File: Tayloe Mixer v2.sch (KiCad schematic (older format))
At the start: 38 parts, among them J1 BNC, J2 Pad, J3 Audio_Jack, J4 Conn_01x04_Female, J5 Pad, T1 6:31, T2 31:6, T3 T50_SPLITTER, U1 LM7805_TO220, U2 FST3253, U3 LM358, U4 si5351, U5 LD33V

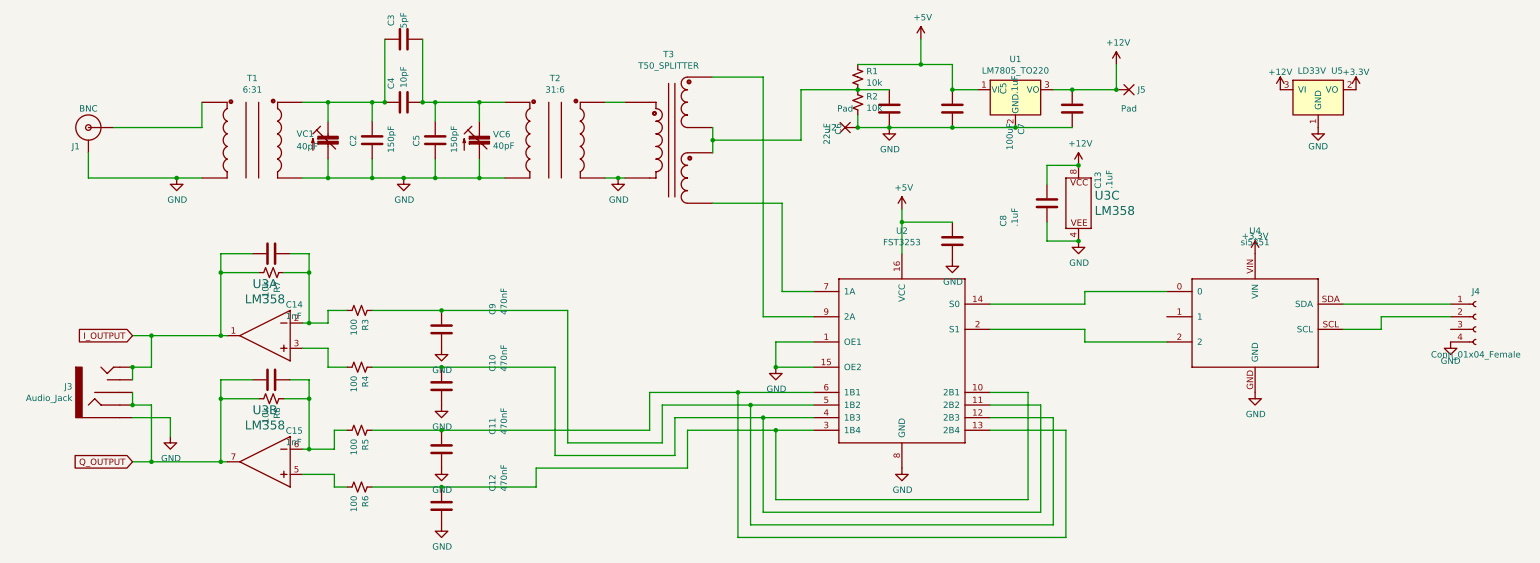
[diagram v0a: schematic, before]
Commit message: gg
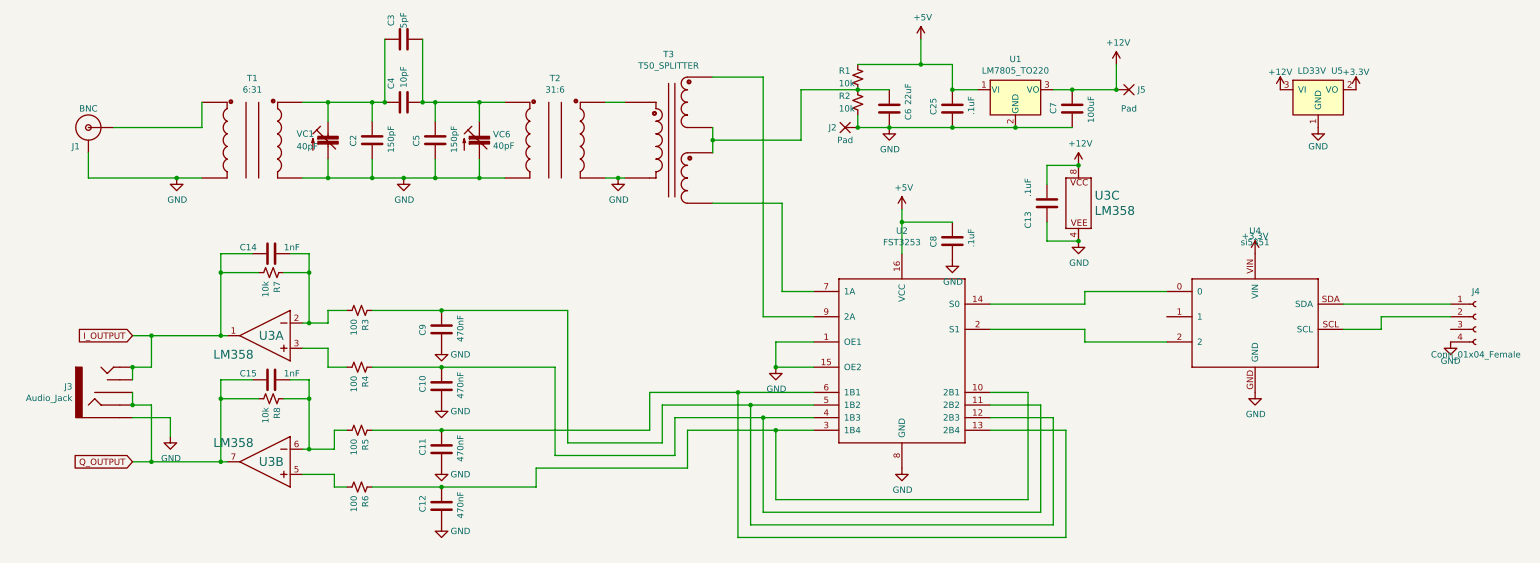
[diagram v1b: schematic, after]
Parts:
- renumbered C5 to C25
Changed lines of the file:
@@
 U 1 1 5E9FAC03
 P 8200 1750
-F 0 "R1" H 8268 1796 50  0000 L CNN
-F 1 "10k" H 8268 1705 50  0000 L CNN
+F 0 "R1" H 8050 1800 50  0000 L CNN
+F 1 "10k" H 8050 1700 50  0000 L CNN
 F 2 "Xenir:Capacitor 0805" H 8200 1750 50  0001 C CNN
 F 3 "~" H 8200 1750 50  0001 C CNN
@@
 U 1 1 5E9FB5EE
 P 8200 1950
-F 0 "R2" H 8268 1996 50  0000 L CNN
-F 1 "10k" H 8268 1905 50  0000 L CNN
+F 0 "R2" H 8050 2000 50  0000 L CNN
+F 1 "10k" H 8050 1900 50  0000 L CNN
 F 2 "Xenir:Capacitor 0805" H 8200 1950 50  0001 C CNN
 F 3 "~" H 8200 1950 50  0001 C CNN
@@
 $EndComp
 $Comp
-L Xenir:Capacitor C5
+L Xenir:Capacitor C25
 U 1 1 5E9FBB07
 P 8950 2000
-F 0 "C5" H 9065 1596 50  0000 L CNN
-F 1 ".1uF" H 9065 1505 50  0000 L CNN
+F 0 "C25" H 8900 2150 50  0000 L CNN
+F 1 ".1uF" H 8900 1850 50  0000 L CNN
 F 2 "Xenir:Capacitor 1206" H 8950 2000 50  0001 C CNN
 F 3 "" H 8950 2000 50  0001 C CNN
@@
 U 1 1 5EA05D6A
 P 9900 2000
-F 0 "C7" H 10015 1596 50  0000 L CNN
-F 1 "100uF" H 10015 1505 50  0000 L CNN
+F 0 "C7" H 9850 1850 50  0000 L CNN
+F 1 "100uF" H 9800 2150 50  0000 L CNN
 F 2 "Capacitor_SMD:CP_Elec_6.3x5.4" H 9900 2000 50  0001 C CNN
 F 3 "" H 9900 2000 50  0001 C CNN
@@
 U 1 1 5EA063C0
 P 8450 2000
-F 0 "C6" H 8565 1596 50  0000 L CNN
-F 1 "22uF" H 8565 1505 50  0000 L CNN
+F 0 "C6" H 8450 2150 50  0000 L CNN
+F 1 "22uF" H 8250 2150 50  0000 L CNN
 F 2 "Capacitor_SMD:CP_Elec_4x5.4" H 8450 2000 50  0001 C CNN
 F 3 "" H 8450 2000 50  0001 C CNN
@@
 U 1 1 5EA383DE
 P 8950 3050
-F 0 "C8" H 9065 2646 50  0000 L CNN
-F 1 ".1uF" H 9065 2555 50  0000 L CNN
+F 0 "C8" H 8900 3200 50  0000 L CNN
+F 1 ".1uF" H 8900 2900 50  0000 L CNN
 F 2 "Xenir:Capacitor 1206" H 8950 3050 50  0001 C CNN
 F 3 "" H 8950 3050 50  0001 C CNN
@@
 U 1 1 5EA6792B
 P 4900 3750
-F 0 "C9" H 5015 3346 50  0000 L CNN
-F 1 "470nF" H 5015 3255 50  0000 L CNN
+F 0 "C9" H 4850 3900 50  0000 L CNN
+F 1 "470nF" H 4800 3600 50  0000 L CNN
 F 2 "Xenir:Capacitor 0805" H 4900 3750 50  0001 C CNN
 F 3 "" H 4900 3750 50  0001 C CNN
@@
 U 1 1 5EA68A05
 P 4900 4200
-F 0 "C10" H 5015 3796 50  0000 L CNN
-F 1 "470nF" H 5015 3705 50  0000 L CNN
+F 0 "C10" H 4850 4350 50  0000 L CNN
+F 1 "470nF" H 4800 4050 50  0000 L CNN
 F 2 "Xenir:Capacitor 0805" H 4900 4200 50  0001 C CNN
 F 3 "" H 4900 4200 50  0001 C CNN
@@
 U 1 1 5EA6950B
 P 4900 4700
-F 0 "C11" H 5015 4296 50  0000 L CNN
-F 1 "470nF" H 5015 4205 50  0000 L CNN
+F 0 "C11" H 4850 4850 50  0000 L CNN
+F 1 "470nF" H 4800 4550 50  0000 L CNN
 F 2 "Xenir:Capacitor 0805" H 4900 4700 50  0001 C CNN
 F 3 "" H 4900 4700 50  0001 C CNN
@@
 U 1 1 5EA69901
 P 4900 5150
-F 0 "C12" H 5015 4746 50  0000 L CNN
-F 1 "470nF" H 5015 4655 50  0000 L CNN
+F 0 "C12" H 4850 5300 50  0000 L CNN
+F 1 "470nF" H 4800 5000 50  0000 L CNN
 F 2 "Xenir:Capacitor 0805" H 4900 5150 50  0001 C CNN
 F 3 "" H 4900 5150 50  0001 C CNN
@@
 P 4900 3900
 F 0 "#PWR05" H 4900 3650 50  0001 C CNN
-F 1 "GND" H 4905 3727 50  0000 C CNN
+F 1 "GND" H 5050 3850 50  0000 C CNN
 F 2 "" H 4900 3900 50  0001 C CNN
 F 3 "" H 4900 3900 50  0001 C CNN
@@
 P 4900 4350
 F 0 "#PWR06" H 4900 4100 50  0001 C CNN
-F 1 "GND" H 4905 4177 50  0000 C CNN
+F 1 "GND" H 5050 4300 50  0000 C CNN
 F 2 "" H 4900 4350 50  0001 C CNN
 F 3 "" H 4900 4350 50  0001 C CNN
@@
 P 4900 4850
 F 0 "#PWR07" H 4900 4600 50  0001 C CNN
-F 1 "GND" H 4905 4677 50  0000 C CNN
+F 1 "GND" H 5050 4800 50  0000 C CNN
 F 2 "" H 4900 4850 50  0001 C CNN
 F 3 "" H 4900 4850 50  0001 C CNN
@@
 P 4900 5300
 F 0 "#PWR08" H 4900 5050 50  0001 C CNN
-F 1 "GND" H 4905 5127 50  0000 C CNN
+F 1 "GND" H 5050 5250 50  0000 C CNN
 F 2 "" H 4900 5300 50  0001 C CNN
 F 3 "" H 4900 5300 50  0001 C CNN
@@
 U 1 1 5EA9F5A6
 P 3500 3800
-F 0 "U3" H 3500 4210 70  0000 C CNN
-F 1 "LM358" H 3500 4089 70  0000 C CNN
+F 0 "U3" H 3450 3800 70  0000 C CNN
+F 1 "LM358" H 3750 3650 70  0000 C CNN
 F 2 "Xenir:SOIC8" H 3450 3750 50  0001 C CNN
 F 3 "" H 3450 3750 50  0001 C CNN
@@
 U 2 1 5EAA17EF
 P 3500 4800
-F 0 "U3" H 3500 5210 70  0000 C CNN
-F 1 "LM358" H 3500 5089 70  0000 C CNN
+F 0 "U3" H 3450 4800 70  0000 C CNN
+F 1 "LM358" H 3750 4950 70  0000 C CNN
 F 2 "Xenir:SOIC8" H 3450 4750 50  0001 C CNN
 F 3 "" H 3450 4750 50  0001 C CNN
@@
 U 1 1 5EAC8FB2
 P 9700 2750
-F 0 "C13" H 9815 2346 50  0000 L CNN
-F 1 ".1uF" H 9815 2255 50  0000 L CNN
+F 0 "C13" H 9500 2900 50  0000 L CNN
+F 1 ".1uF" H 9750 2900 50  0000 L CNN
 F 2 "Xenir:Capacitor 1206" H 9700 2750 50  0001 C CNN
 F 3 "" H 9700 2750 50  0001 C CNN
@@
 U 1 1 5EADF0CD
 P 3550 4150
-F 0 "C15" H 3665 3746 50  0000 L CNN
-F 1 "1nF" H 3665 3655 50  0000 L CNN
+F 0 "C15" H 3300 4200 50  0000 L CNN
+F 1 "1nF" H 3650 4200 50  0000 L CNN
 F 2 "Xenir:Capacitor 0805" H 3550 4150 50  0001 C CNN
 F 3 "" H 3550 4150 50  0001 C CNN
@@
 U 1 1 5EADE1CD
 P 3550 3150
-F 0 "C14" H 3665 2746 50  0000 L CNN
-F 1 "1nF" H 3665 2655 50  0000 L CNN
+F 0 "C14" H 3300 3200 50  0000 L CNN
+F 1 "1nF" H 3650 3200 50  0000 L CNN
 F 2 "Xenir:Capacitor 0805" H 3550 3150 50  0001 C CNN
 F 3 "" H 3550 3150 50  0001 C CNN
@@
 P 8100 2000
 F 0 "J2" H 8000 1850 50  0000 C CNN
-F 1 "Pad" H 8100 2000 50  0000 C CNN
+F 1 "Pad" H 8100 1750 50  0000 C CNN
 F 2 "Xenir:Pad" H 8100 2000 50  0001 C CNN
 F 3 "" H 8100 2000 50  0001 C CNN

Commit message: gg
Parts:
- R1, R2, R3, R4, R5, R6, R7, R8: footprint Xenir:Capacitor 0805 -> Xenir:Resistor 0805
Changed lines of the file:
@@
 F 0 "R1" H 8050 1800 50  0000 L CNN
 F 1 "10k" H 8050 1700 50  0000 L CNN
-F 2 "Xenir:Capacitor 0805" H 8200 1750 50  0001 C CNN
+F 2 "Xenir:Resistor 0805" H 8200 1750 50  0001 C CNN
 F 3 "~" H 8200 1750 50  0001 C CNN
 	1    8200 1750
@@
 F 0 "R2" H 8050 2000 50  0000 L CNN
 F 1 "10k" H 8050 1900 50  0000 L CNN
-F 2 "Xenir:Capacitor 0805" H 8200 1950 50  0001 C CNN
+F 2 "Xenir:Resistor 0805" H 8200 1950 50  0001 C CNN
 F 3 "~" H 8200 1950 50  0001 C CNN
 	1    8200 1950
@@
 F 0 "R3" H 4318 3646 50  0000 L CNN
 F 1 "100" H 4318 3555 50  0000 L CNN
-F 2 "Xenir:Capacitor 0805" H 4250 3600 50  0001 C CNN
+F 2 "Xenir:Resistor 0805" H 4250 3600 50  0001 C CNN
 F 3 "~" H 4250 3600 50  0001 C CNN
 	1    4250 3600
@@
 F 0 "R4" H 4318 4096 50  0000 L CNN
 F 1 "100" H 4318 4005 50  0000 L CNN
-F 2 "Xenir:Capacitor 0805" H 4250 4050 50  0001 C CNN
+F 2 "Xenir:Resistor 0805" H 4250 4050 50  0001 C CNN
 F 3 "~" H 4250 4050 50  0001 C CNN
 	1    4250 4050
@@
 F 0 "R5" H 4318 4596 50  0000 L CNN
 F 1 "100" H 4318 4505 50  0000 L CNN
-F 2 "Xenir:Capacitor 0805" H 4250 4550 50  0001 C CNN
+F 2 "Xenir:Resistor 0805" H 4250 4550 50  0001 C CNN
 F 3 "~" H 4250 4550 50  0001 C CNN
 	1    4250 4550
@@
 F 0 "R6" H 4318 5046 50  0000 L CNN
 F 1 "100" H 4318 4955 50  0000 L CNN
-F 2 "Xenir:Capacitor 0805" H 4250 5000 50  0001 C CNN
+F 2 "Xenir:Resistor 0805" H 4250 5000 50  0001 C CNN
 F 3 "~" H 4250 5000 50  0001 C CNN
 	1    4250 5000
@@
 F 0 "R7" H 3618 3346 50  0000 L CNN
 F 1 "10k" H 3618 3255 50  0000 L CNN
-F 2 "Xenir:Capacitor 0805" H 3550 3300 50  0001 C CNN
+F 2 "Xenir:Resistor 0805" H 3550 3300 50  0001 C CNN
 F 3 "~" H 3550 3300 50  0001 C CNN
 	1    3550 3300
@@
 F 0 "R8" H 3618 4346 50  0000 L CNN
 F 1 "10k" H 3618 4255 50  0000 L CNN
-F 2 "Xenir:Capacitor 0805" H 3550 4300 50  0001 C CNN
+F 2 "Xenir:Resistor 0805" H 3550 4300 50  0001 C CNN
 F 3 "~" H 3550 4300 50  0001 C CNN
 	1    3550 4300

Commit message: rescue
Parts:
- C10, C11, C12, C13, C14, C15, C2, C25, C3, C4, C5, C6, C7, C8, C9: symbol Xenir:Capacitor -> Tayloe-Mixer-v2-rescue:Capacitor-Xenir
- J1: symbol Xenir:BNC -> Tayloe-Mixer-v2-rescue:BNC-Xenir
- J2, J5: symbol Xenir:Pad -> Tayloe-Mixer-v2-rescue:Pad-Xenir
- J3: symbol Xenir:Audio_Jack -> Tayloe-Mixer-v2-rescue:Audio_Jack-Xenir
- T1, T2: symbol Xenir:T37_XFRM -> Tayloe-Mixer-v2-rescue:T37_XFRM-Xenir
- T3: symbol Xenir:T50_SPLITTER -> Tayloe-Mixer-v2-rescue:T50_SPLITTER-Xenir
- U2: symbol Xenir:FST3253 -> Tayloe-Mixer-v2-rescue:FST3253-Xenir
- U3: symbol Xenir:LM358 -> Tayloe-Mixer-v2-rescue:LM358-Xenir
- U4: symbol Xenir:si5351 -> Tayloe-Mixer-v2-rescue:si5351-Xenir
- U5: symbol Xenir:LD33V -> Tayloe-Mixer-v2-rescue:LD33V-Xenir
- VC1, VC6: symbol Xenir:Trimcap -> Tayloe-Mixer-v2-rescue:Trimcap-Xenir
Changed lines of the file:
@@
 $EndComp
 $Comp
-L Xenir:Capacitor C25
+L Tayloe-Mixer-v2-rescue:Capacitor-Xenir C25
 U 1 1 5E9FBB07
 P 8950 2000
@@
 	7750 1850 8200 1850
 $Comp
-L Xenir:Capacitor C7
+L Tayloe-Mixer-v2-rescue:Capacitor-Xenir C7
 U 1 1 5EA05D6A
 P 9900 2000
@@
 $EndComp
 $Comp
-L Xenir:Capacitor C6
+L Tayloe-Mixer-v2-rescue:Capacitor-Xenir C6
 U 1 1 5EA063C0
 P 8450 2000
@@
 	8700 1650 8950 1650
 $Comp
-L Xenir:FST3253 U2
+L Tayloe-Mixer-v2-rescue:FST3253-Xenir U2
 U 1 1 5EA318D2
 P 9000 2700
@@
 	8550 2800 8550 2900
 $Comp
-L Xenir:Capacitor C8
+L Tayloe-Mixer-v2-rescue:Capacitor-Xenir C8
 U 1 1 5EA383DE
 P 8950 3050
@@
 	9550 4250 9250 4250
 $Comp
-L Xenir:Capacitor C9
+L Tayloe-Mixer-v2-rescue:Capacitor-Xenir C9
 U 1 1 5EA6792B
 P 4900 3750
@@
 $EndComp
 $Comp
-L Xenir:Capacitor C10
+L Tayloe-Mixer-v2-rescue:Capacitor-Xenir C10
 U 1 1 5EA68A05
 P 4900 4200
@@
 $EndComp
 $Comp
-L Xenir:Capacitor C11
+L Tayloe-Mixer-v2-rescue:Capacitor-Xenir C11
 U 1 1 5EA6950B
 P 4900 4700
@@
 $EndComp
 $Comp
-L Xenir:Capacitor C12
+L Tayloe-Mixer-v2-rescue:Capacitor-Xenir C12
 U 1 1 5EA69901
 P 4900 5150
@@
 $EndComp
 $Comp
-L Xenir:LM358 U3
+L Tayloe-Mixer-v2-rescue:LM358-Xenir U3
 U 1 1 5EA9F5A6
 P 3500 3800
@@
 $EndComp
 $Comp
-L Xenir:LM358 U3
+L Tayloe-Mixer-v2-rescue:LM358-Xenir U3
 U 2 1 5EAA17EF
 P 3500 4800
@@
 $EndComp
 $Comp
-L Xenir:LM358 U3
+L Tayloe-Mixer-v2-rescue:LM358-Xenir U3
 U 3 1 5EAA2951
 P 10050 2750
@@
 $EndComp
 $Comp
-L Xenir:Capacitor C13
+L Tayloe-Mixer-v2-rescue:Capacitor-Xenir C13
 U 1 1 5EAC8FB2
 P 9700 2750
@@
 $EndComp
 $Comp
-L Xenir:Capacitor C15
+L Tayloe-Mixer-v2-rescue:Capacitor-Xenir C15
 U 1 1 5EADF0CD
 P 3550 4150
@@
 	3850 4300 3850 4700
 $Comp
-L Xenir:Capacitor C14
+L Tayloe-Mixer-v2-rescue:Capacitor-Xenir C14
 U 1 1 5EADE1CD
 P 3550 3150
@@
 	6200 1950 6350 1950
 $Comp
-L Xenir:T50_SPLITTER T3
+L Tayloe-Mixer-v2-rescue:T50_SPLITTER-Xenir T3
 U 1 1 5E9EEE06
 P 6700 1550
@@
 	4750 1950 4850 1950
 $Comp
-L Xenir:T37_XFRM T2
+L Tayloe-Mixer-v2-rescue:T37_XFRM-Xenir T2
 U 1 1 5E9E9ADC
 P 5800 1800
@@
 $EndComp
 $Comp
-L Xenir:Trimcap VC6
+L Tayloe-Mixer-v2-rescue:Trimcap-Xenir VC6
 U 1 1 5E9E8F97
 P 5200 1850
@@
 $EndComp
 $Comp
-L Xenir:Capacitor C3
+L Tayloe-Mixer-v2-rescue:Capacitor-Xenir C3
 U 1 1 5E9E8D24
 P 4600 1450
@@
 $EndComp
 $Comp
-L Xenir:Capacitor C4
+L Tayloe-Mixer-v2-rescue:Capacitor-Xenir C4
 U 1 1 5E9E81AF
 P 4600 1950
@@
 $EndComp
 $Comp
-L Xenir:Capacitor C5
+L Tayloe-Mixer-v2-rescue:Capacitor-Xenir C5
 U 1 1 5E9E7736
 P 4850 2250
@@
 $EndComp
 $Comp
-L Xenir:Capacitor C2
+L Tayloe-Mixer-v2-rescue:Capacitor-Xenir C2
 U 1 1 5E9E667F
 P 4350 2250
@@
 $EndComp
 $Comp
-L Xenir:Trimcap VC1
+L Tayloe-Mixer-v2-rescue:Trimcap-Xenir VC1
 U 1 1 5E9DC9D6
 P 4000 1850
@@
 	3000 2150 3000 1950
 $Comp
-L Xenir:T37_XFRM T1
+L Tayloe-Mixer-v2-rescue:T37_XFRM-Xenir T1
 U 1 1 5E9D7159
 P 3400 1800
@@
 Connection ~ 3150 4800
 $Comp
-L Xenir:si5351 U4
+L Tayloe-Mixer-v2-rescue:si5351-Xenir U4
 U 1 1 5E9EA10D
 P 11600 3250
@@
 $EndComp
 $Comp
-L Xenir:Audio_Jack J3
+L Tayloe-Mixer-v2-rescue:Audio_Jack-Xenir J3
 U 1 1 5E9E7BEE
 P 2250 4600
@@
 	10000 3750 9250 3750
 $Comp
-L Xenir:BNC J1
+L Tayloe-Mixer-v2-rescue:BNC-Xenir J1
 U 1 1 5F44E5DC
 P 2100 2150
@@
 $EndComp
 $Comp
-L Xenir:LD33V U5
+L Tayloe-Mixer-v2-rescue:LD33V-Xenir U5
 U 1 1 5F4A2EFF
 P 11850 1700
@@
 Connection ~ 2450 4350
 $Comp
-L Xenir:Pad J5
+L Tayloe-Mixer-v2-rescue:Pad-Xenir J5
 U 1 1 5F486548
 P 10350 2000
@@
 Connection ~ 10250 1850
 $Comp
-L Xenir:Pad J2
+L Tayloe-Mixer-v2-rescue:Pad-Xenir J2
 U 1 1 5F4876B8
 P 8100 2000
